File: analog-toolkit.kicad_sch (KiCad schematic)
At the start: 52 parts, among them J1 USB_C, J2 IO, J3 UART, J4 I2C, J5 VBUS, J6 3.3V, J7 OPAMP, J8 ADC, P1 TC2030, SW1 DFU, U1 AP2204R-3.3, U2 otter_USBLC6-4, U3 STM32G431KBT6

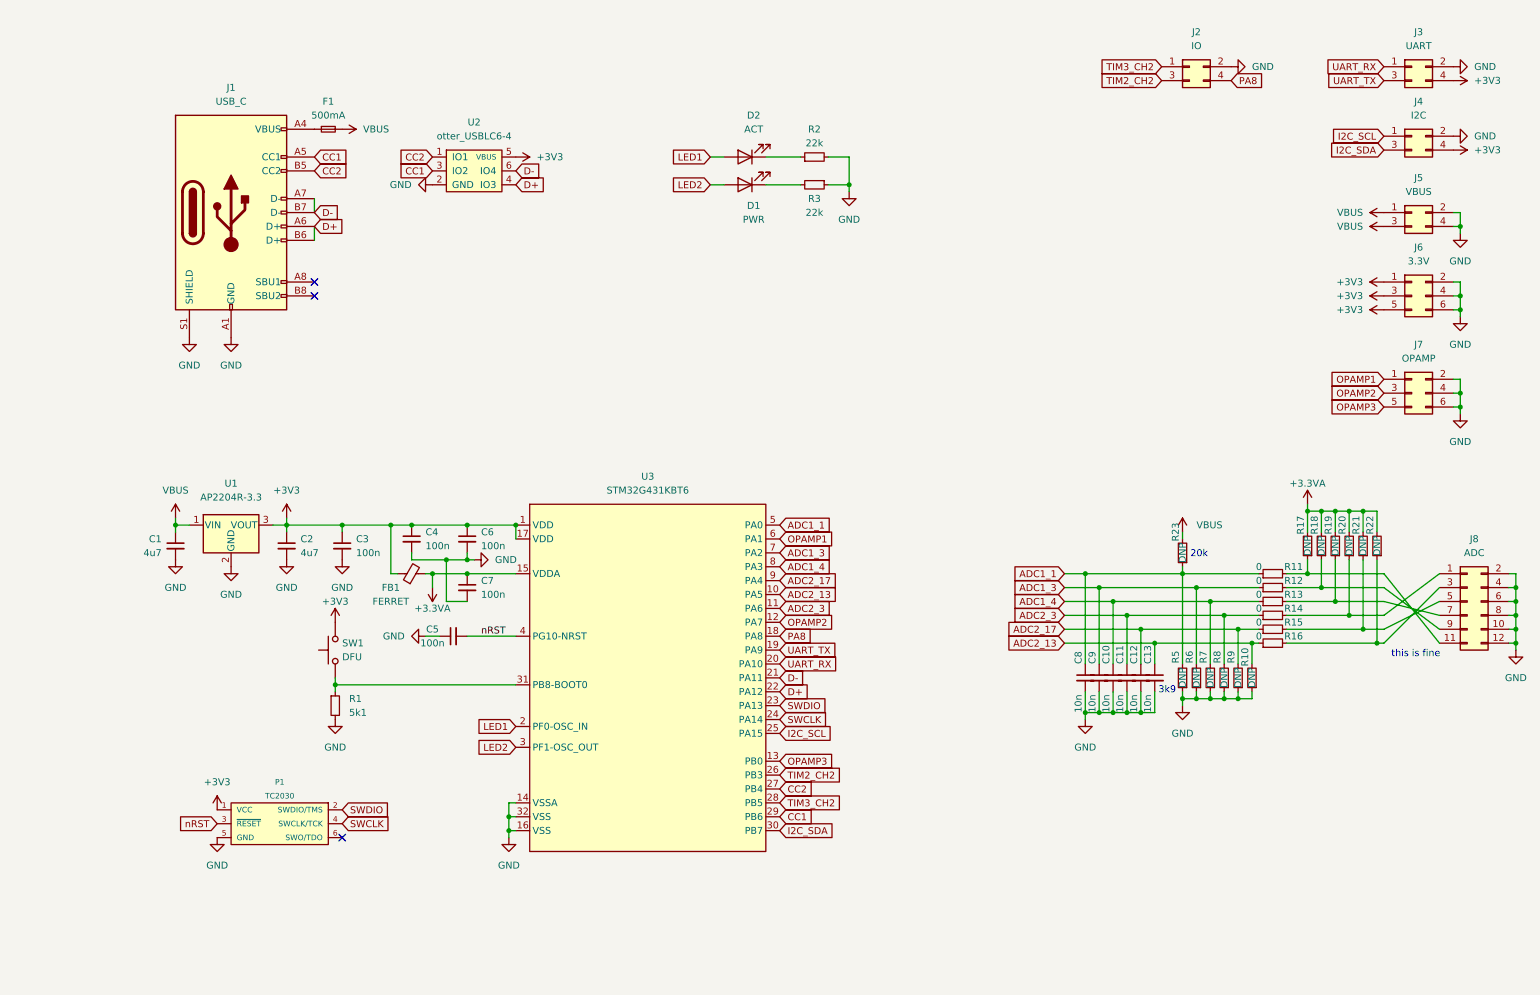
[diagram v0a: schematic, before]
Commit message: added r3
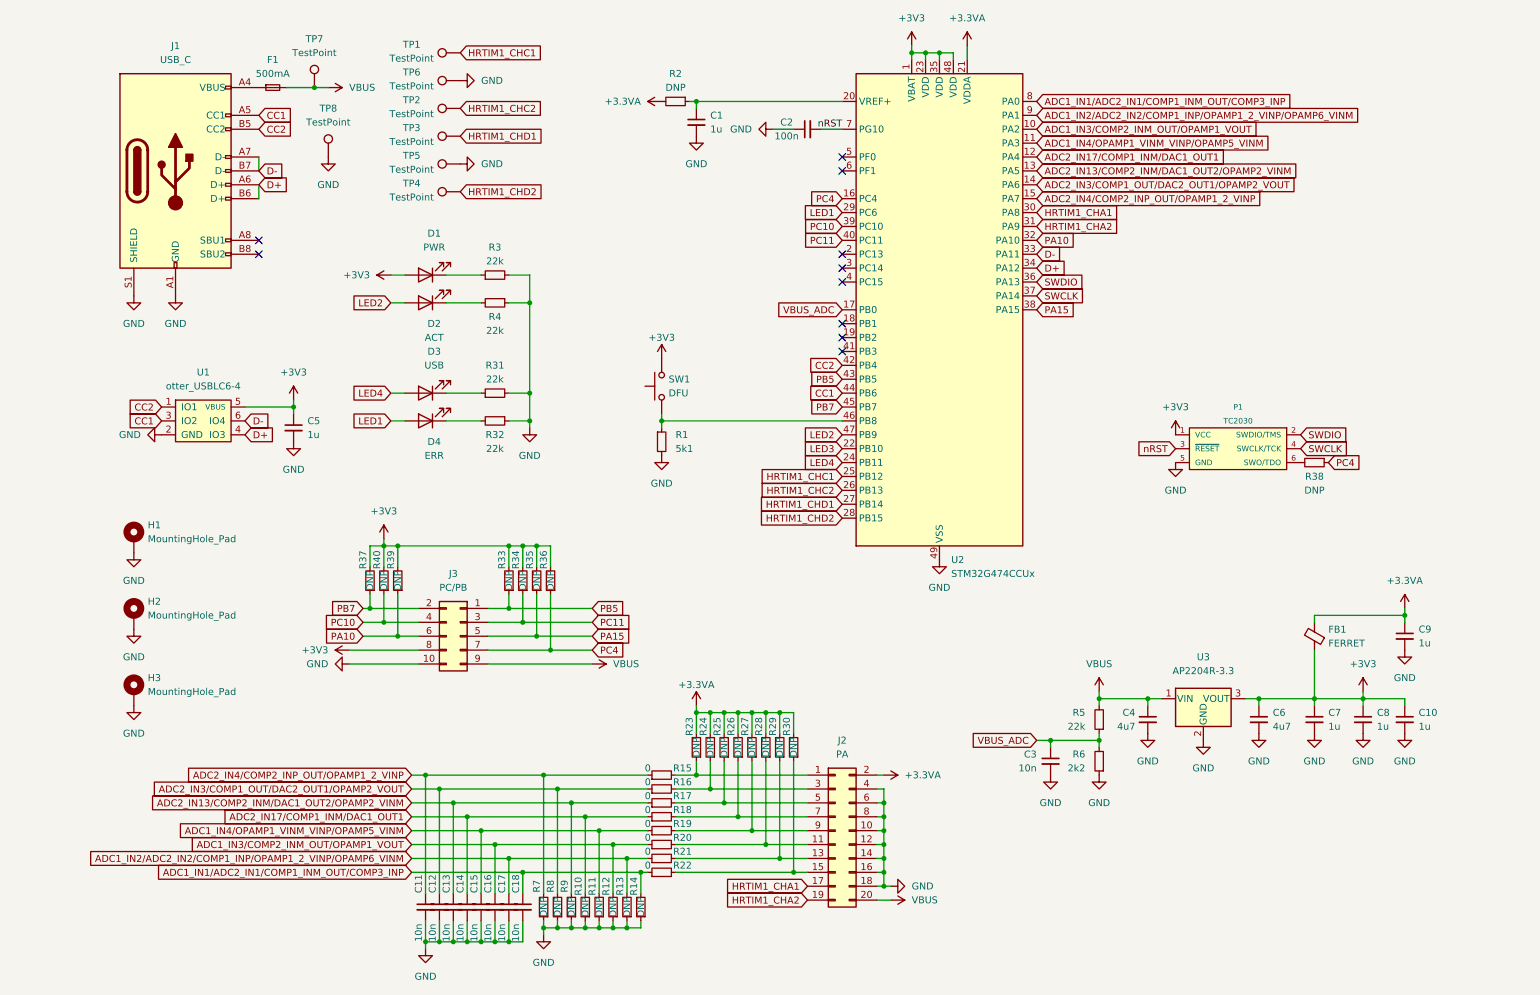
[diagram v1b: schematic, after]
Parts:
- removed C6: 100n, otter:C_0402, symbol Device:C_Small
- removed J2: IO, Connector_PinHeader_2.54mm:PinHeader_2x02_P2.54mm_Horizontal, symbol Connector_Generic:Conn_02x02_Odd_Even
- removed J3: UART, Connector_PinHeader_2.54mm:PinHeader_2x02_P2.54mm_Horizontal, symbol Connector_Generic:Conn_02x02_Odd_Even
- removed J4: I2C, Connector_PinHeader_2.54mm:PinHeader_2x02_P2.54mm_Horizontal, symbol Connector_Generic:Conn_02x02_Odd_Even
- removed J5: VBUS, Connector_PinHeader_2.54mm:PinHeader_2x02_P2.54mm_Horizontal, symbol Connector_Generic:Conn_02x02_Odd_Even
- removed J6: 3.3V, Connector_PinHeader_2.54mm:PinHeader_2x03_P2.54mm_Horizontal, symbol Connector_Generic:Conn_02x03_Odd_Even
- removed J7: OPAMP, Connector_PinHeader_2.54mm:PinHeader_2x03_P2.54mm_Horizontal, symbol Connector_Generic:Conn_02x03_Odd_Even
- removed J8: ADC, Connector_PinHeader_2.54mm:PinHeader_2x06_P2.54mm_Horizontal, symbol Connector_Generic:Conn_02x06_Odd_Even
- removed U3: STM32G431KBT6, Package_QFP:LQFP-32_7x7mm_P0.8mm, symbol otter:STM32G431xB
- added C14, C15, C16, C17, C18: 10n, otter:C_0402, symbol Device:C_Small
- added C5: 1u, otter:C_0402, symbol Device:C_Small
- added D3: USB, LED_SMD:LED_0805_2012Metric, symbol Device:LED
- added D4: ERR, LED_SMD:LED_0805_2012Metric, symbol Device:LED
- added H1, H2, H3: MountingHole_Pad, MountingHole:MountingHole_2.2mm_M2_ISO7380_Pad, symbol Mechanical:MountingHole_Pad
- added J2: PA, Connector_IDC:IDC-Header_2x10_P2.54mm_Horizontal, symbol Connector_Generic:Conn_02x10_Odd_Even
- added J3: PC/PB, Connector_IDC:IDC-Header_2x05_P2.54mm_Horizontal, symbol Connector_Generic:Conn_02x05_Odd_Even
- added R2, R24, R25, R26, R27, R28, R29, R30, R33, R34, R35, R36, R37, R38, R39, R40: DNP, otter:R_0402, symbol Device:R_Small
- added R31, R32: 22k, otter:R_0402, symbol Device:R_Small
- added TP1, TP2, TP3, TP4, TP5, TP6, TP7, TP8: TestPoint, TestPoint:TestPoint_Pad_1.0x1.0mm, symbol Connector:TestPoint
- added U2: STM32G474CCUx, Package_DFN_QFN:QFN-48-1EP_7x7mm_P0.5mm_EP5.6x5.6mm, symbol MCU_ST_STM32G4:STM32G474CCUx
- C1: value 4u7 -> 1u; footprint otter:C_0603 -> otter:C_0402; lcsc (none) -> C52923
- C10, C8, C9: value 10n -> 1u; lcsc (none) -> C52923
- C11, C12, C13: lcsc (none) -> C15195
- C3: value 100n -> 10n; lcsc (none) -> C15195
- C4: value 100n -> 4u7; footprint otter:C_0402 -> otter:C_0805; lcsc (none) -> C1779
- C6: renamed from C2; footprint otter:C_0603 -> otter:C_0805; lcsc (none) -> C1779
- C7: value 100n -> 1u; lcsc (none) -> C52923
- D1: renamed from D2; value ACT -> PWR
- D2: renamed from D1; value PWR -> ACT
- FB1: lcsc (none) -> C1002
- R11, R12, R13, R14: value 0 -> DNP
- R15, R16: lcsc (none) -> C17168
- R17, R18, R19, R20, R21, R22: value DNP -> 0; lcsc (none) -> C17168
- R5: value DNP -> 22k; lcsc (none) -> C25768
- R6: value DNP -> 2k2; lcsc (none) -> C25890
- renumbered C5 to C2, R2 to R3, R3 to R4, U2 to U1, U1 to U3
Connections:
- net +3.3VA: now also C9.1, R23.2, J2.2 (Pin_2), R2.2, R24.2, R25.2, R26.2, R27.2, R28.2, R29.2, R30.2, U2.21 (VDDA); no longer C7.1, R17.2, R18.2, R19.2, R20.2, R21.2, R22.2
- net +3V3: now also C10.1, C7.1, C8.1, D1.2 (A), C5.1, J3.8 (Pin_8), R33.2, R34.2, R35.2, R36.2, R37.2, R39.2, R40.2, U2.1 (VBAT), U2.23 (VDD), U2.35 (VDD), U2.48 (VDD); no longer C3.1, C4.1
- net CC1: now also U2.44 (PB6)
- net CC2: now also U2.42 (PB4)
- net D+: now also U2.34 (PA12)
- net D-: now also U2.33 (PA11)
- net GND: now also R11.1, R12.1, R13.1, R14.1, C14.2, C15.2, C16.2, C17.2, C18.2, C5.2, H1.1, H2.1, H3.1, J2.10 (Pin_10), J2.12 (Pin_12), J2.14 (Pin_14), J2.16 (Pin_16), J2.18 (Pin_18), J2.4 (Pin_4), J2.6 (Pin_6), J2.8 (Pin_8), J3.10 (Pin_10), R31.2, R32.1, TP5.1, TP6.1, TP8.1, U2.49 (VSS); no longer R5.1
- net LED1: now also D4.2 (A), U2.29 (PC6); no longer D1.2 (A)
- net LED2: now also U2.47 (PB9)
- net SWCLK: now also U2.37 (PA14)
- net SWDIO: now also U2.36 (PA13)
- net VBUS: now also C4.1, R5.2, J2.20 (Pin_20), J3.9 (Pin_9), TP7.1; no longer C1.1, R23.2
- net nRST: now also U2.7 (PG10)
- net at R15.2: now also R23.1, J2.1 (Pin_1); no longer R21.1
- net at R1.1, SW1.1: now also U2.46 (PB8)
- net at R16.2: now also J2.3 (Pin_3), R24.1; no longer R22.1
- net at P1.6 (SWO/TDO): now also R38.2
- net ADC1_IN2/ADC2_IN2/COMP1_INP/OPAMP1_2_VINP/OPAMP6_VINM: now reaches R13.2
- net ADC1_IN2/ADC2_IN2/COMP1_INP/OPAMP1_2_VINP/OPAMP6_VINM: now also R21.1, C17.1, U2.9 (PA1); no longer R19.1
- net ADC1_IN4/OPAMP1_VINM_VINP/OPAMP5_VINM: now reaches R11.2
- net ADC1_IN4/OPAMP1_VINM_VINP/OPAMP5_VINM: now also R19.1, C15.1, U2.11 (PA3); no longer R17.1
- net ADC1_IN1/ADC2_IN1/COMP1_INM_OUT/COMP3_INP: now reaches R14.2
- net ADC1_IN1/ADC2_IN1/COMP1_INM_OUT/COMP3_INP: now also R22.1, C18.1, U2.8 (PA0); no longer R20.1
- net ADC1_IN3/COMP2_INM_OUT/OPAMP1_VOUT: now reaches R12.2
- net ADC1_IN3/COMP2_INM_OUT/OPAMP1_VOUT: now also R20.1, C16.1, U2.10 (PA2); no longer R18.1
- removed net ADC1_1: C8.1, R11.1, R23.1, R5.2
- removed net ADC1_3: C9.1, R12.1, R6.2
- removed net ADC1_4: C10.1, R13.1, R7.2
- removed net ADC2_13: C13.1, R10.2, R16.1
- removed net ADC2_17: C12.1, R15.1, R9.2
- removed net ADC2_3: C11.1, R14.1, R8.2
- new net: J2.9 (Pin_9), R19.2, R27.1
- new net: D4.1 (K), R32.2
- new net: J2.11 (Pin_11), R20.2, R28.1
- new net: J2.13 (Pin_13), R21.2, R29.1
- new net: J2.15 (Pin_15), R22.2, R30.1
- new net: J2.5 (Pin_5), R17.2, R25.1
- new net: J2.7 (Pin_7), R18.2, R26.1
- new net: C1.1, R2.1, U2.20 (VREF+)
- new net: D3.1 (K), R31.1
- new net ADC2_IN13/COMP2_INM/DAC1_OUT2/OPAMP2_VINM: C13.1, R17.1, R9.2, U2.13 (PA5)
- new net ADC2_IN17/COMP1_INM/DAC1_OUT1: C14.1, R10.2, R18.1, U2.12 (PA4)
- new net ADC2_IN3/COMP1_OUT/DAC2_OUT1/OPAMP2_VOUT: C12.1, R16.1, R8.2, U2.14 (PA6)
- new net ADC2_IN4/COMP2_INP_OUT/OPAMP1_2_VINP: C11.1, R15.1, R7.2, U2.15 (PA7)
- new net HRTIM1_CHA1: J2.17 (Pin_17), U2.30 (PA8)
- new net HRTIM1_CHA2: J2.19 (Pin_19), U2.31 (PA9)
- new net HRTIM1_CHC1: TP1.1, U2.25 (PB12)
- new net HRTIM1_CHC2: TP2.1, U2.26 (PB13)
- new net HRTIM1_CHD1: TP3.1, U2.27 (PB14)
- new net HRTIM1_CHD2: TP4.1, U2.28 (PB15)
- new net LED3: U2.22 (PB10)
- new net LED4: D3.2 (A), U2.24 (PB11)
- new net PA10: J3.6 (Pin_6), R39.1, U2.32 (PA10)
- new net PA15: J3.5 (Pin_5), R35.1, U2.38 (PA15)
- new net PB5: J3.1 (Pin_1), R33.1, U2.43 (PB5)
- new net PB7: J3.2 (Pin_2), R37.1, U2.45 (PB7)
- new net PC10: J3.4 (Pin_4), R40.1, U2.39 (PC10)
- new net PC11: J3.3 (Pin_3), R34.1, U2.40 (PC11)
- new net PC4: J3.7 (Pin_7), R36.1, R38.1, U2.16 (PC4)
- new net VBUS_ADC: C3.1, R5.1, R6.2, U2.17 (PB0)
- no-connect marks 3 -> 10
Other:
- note removed: "20k"
- note removed: "3k9"
- note removed: "this is fine"
- company: Jana Hemsing -> Jana M. Hemsing
- moved on the sheet: C2, C6, D1, D2, F1, FB1, J1, P1, R1, R3, R4, SW1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
